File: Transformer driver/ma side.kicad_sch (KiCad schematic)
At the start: 23 parts, among them Q1 NPN, Q3 NPN, Q4 PNP, Q5 PNP, Q6 IRF540N, Q7 IRF540N, U5 IR2153

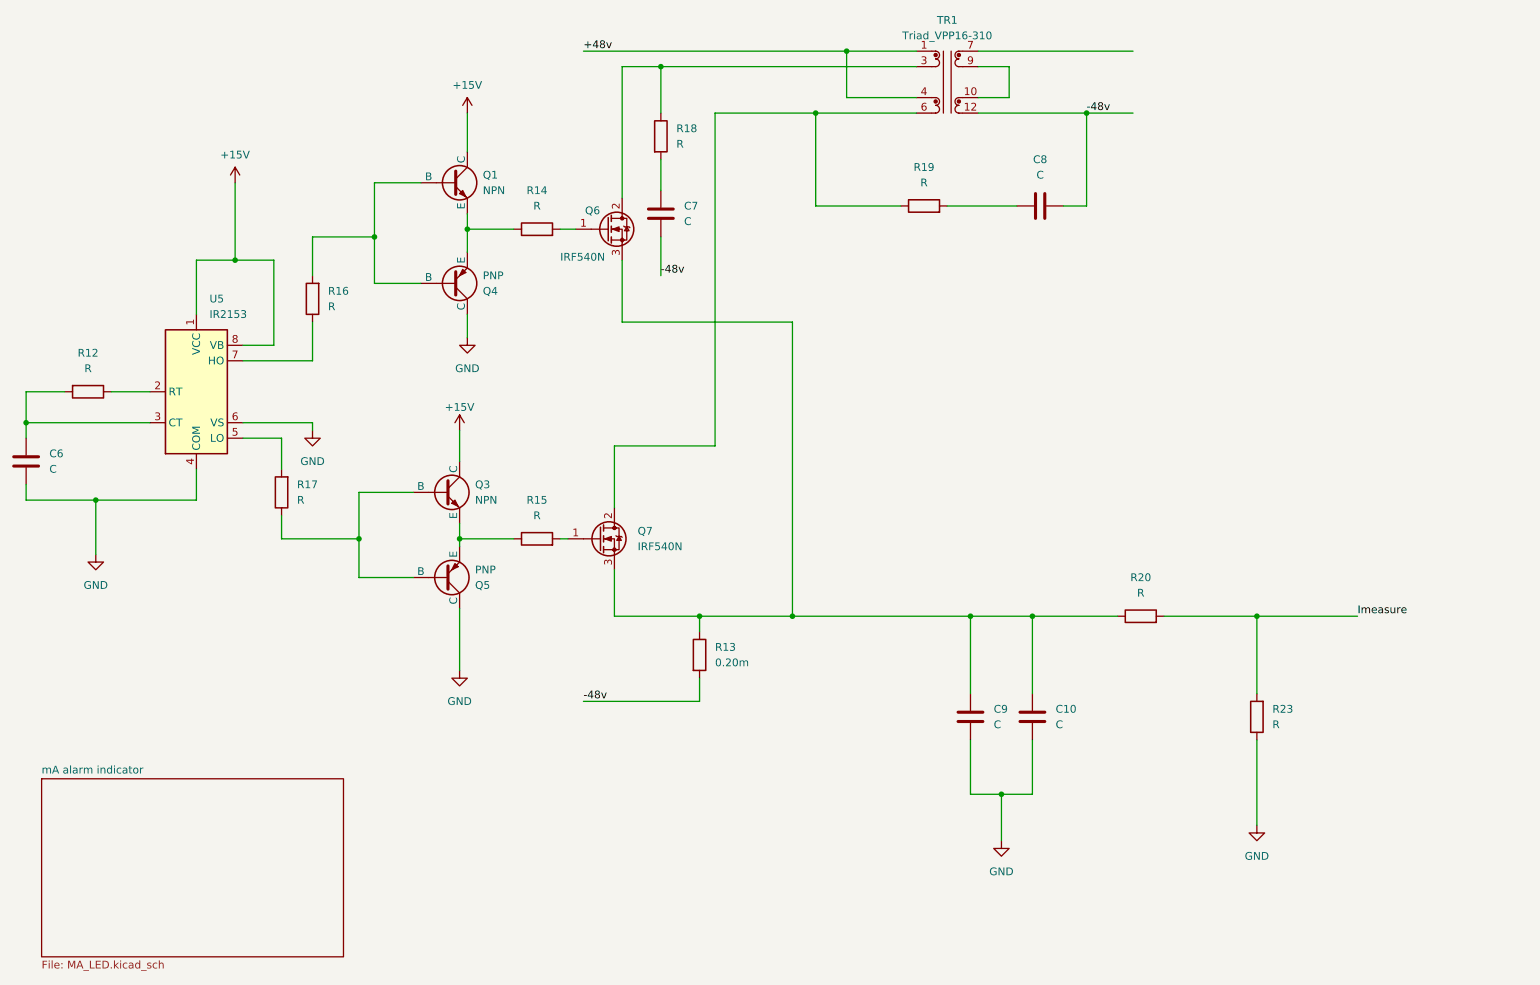
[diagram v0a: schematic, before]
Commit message: commit
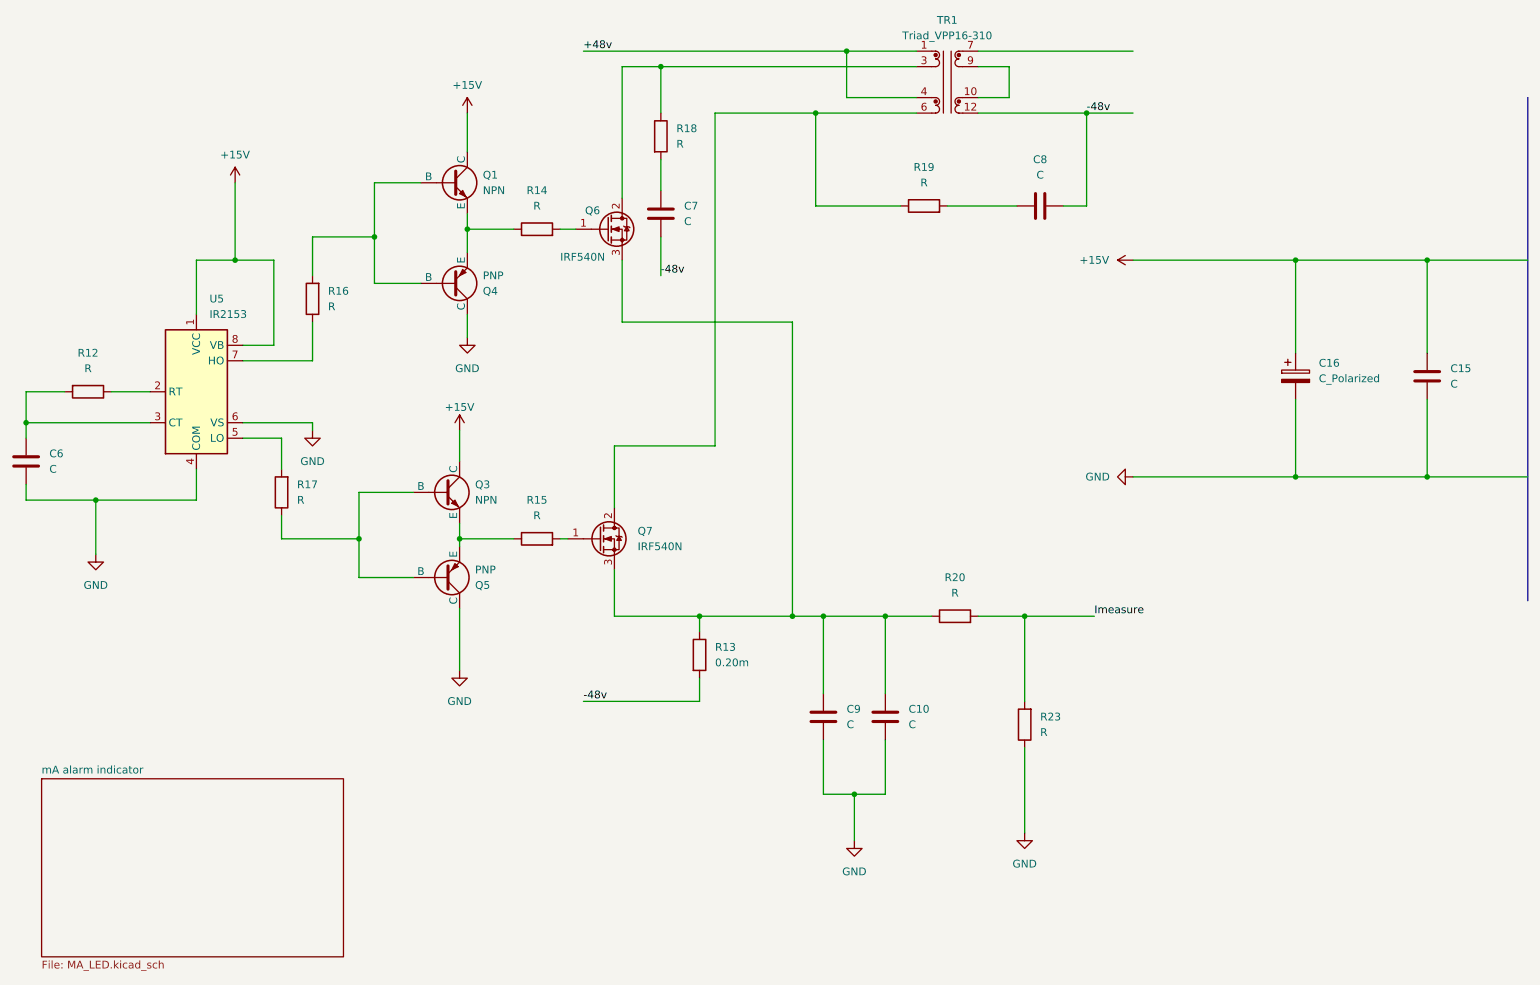
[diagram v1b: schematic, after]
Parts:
- added C15: C, symbol Device:C
- added C16: C_Polarized, symbol Device:C_Polarized
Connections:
- net +15V: now also C15.1, C16.1
- net GND: now also C15.2, C16.2
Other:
- moved on the sheet: C10, C9, R20, R23
